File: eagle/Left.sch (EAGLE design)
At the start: 4 parts, among them J1 Rows, J2 Columns

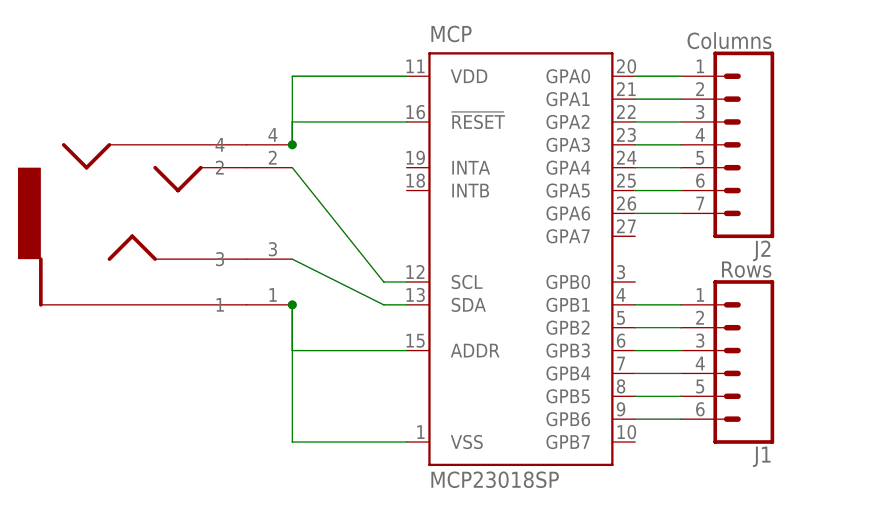
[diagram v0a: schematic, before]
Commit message: v03 of Left board
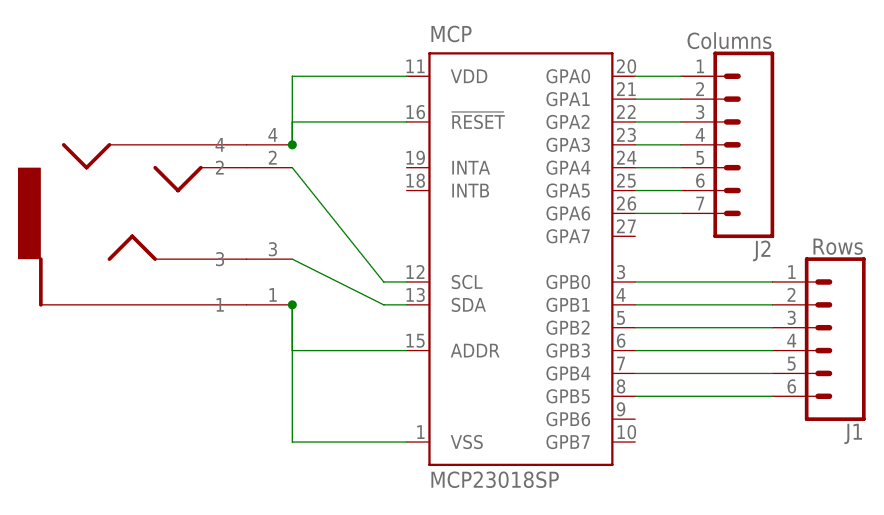
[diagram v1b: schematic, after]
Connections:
- net N$12: now also MCP.GPB0; no longer MCP.GPB1
- net N$13: now also MCP.GPB1; no longer MCP.GPB2
- net N$14: now also MCP.GPB2; no longer MCP.GPB3
- net N$15: now also MCP.GPB3; no longer MCP.GPB4
- net N$16: now also MCP.GPB4; no longer MCP.GPB5
- net N$17: now also MCP.GPB5; no longer MCP.GPB6
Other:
- moved on the sheet: J1
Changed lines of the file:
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@@
 <instance part="MCP" gate="G$1" x="25.4" y="162.56"/>
 <instance part="J2" gate="G$1" x="48.26" y="177.8" rot="R180"/>
-<instance part="J1" gate="G$1" x="48.26" y="152.4" rot="R180"/>
+<instance part="J1" gate="G$1" x="58.42" y="154.94" rot="R180"/>
 </instances>
 <busses>
@@
 <net name="N$12" class="0">
 <segment>
-<pinref part="MCP" gate="G$1" pin="GPB1"/>
+<pinref part="MCP" gate="G$1" pin="GPB0"/>
 <pinref part="J1" gate="G$1" pin="1"/>
-<wire x1="38.1" y1="157.48" x2="43.18" y2="157.48" width="0.1524" layer="91"/>
+<wire x1="38.1" y1="160.02" x2="53.34" y2="160.02" width="0.1524" layer="91"/>
 </segment>
 </net>
 <net name="N$13" class="0">
 <segment>
-<pinref part="MCP" gate="G$1" pin="GPB2"/>
+<pinref part="MCP" gate="G$1" pin="GPB1"/>
 <pinref part="J1" gate="G$1" pin="2"/>
-<wire x1="38.1" y1="154.94" x2="43.18" y2="154.94" width="0.1524" layer="91"/>
+<wire x1="38.1" y1="157.48" x2="53.34" y2="157.48" width="0.1524" layer="91"/>
 </segment>
 </net>
 <net name="N$14" class="0">
 <segment>
-<pinref part="MCP" gate="G$1" pin="GPB3"/>
+<pinref part="MCP" gate="G$1" pin="GPB2"/>
 <pinref part="J1" gate="G$1" pin="3"/>
-<wire x1="38.1" y1="152.4" x2="43.18" y2="152.4" width="0.1524" layer="91"/>
+<wire x1="38.1" y1="154.94" x2="53.34" y2="154.94" width="0.1524" layer="91"/>
 </segment>
 </net>
 <net name="N$15" class="0">
 <segment>
-<pinref part="MCP" gate="G$1" pin="GPB4"/>
+<pinref part="MCP" gate="G$1" pin="GPB3"/>
 <pinref part="J1" gate="G$1" pin="4"/>
-<wire x1="38.1" y1="149.86" x2="43.18" y2="149.86" width="0.1524" layer="91"/>
+<wire x1="38.1" y1="152.4" x2="53.34" y2="152.4" width="0.1524" layer="91"/>
 </segment>
 </net>
 <net name="N$16" class="0">
 <segment>
-<pinref part="MCP" gate="G$1" pin="GPB5"/>
+<pinref part="MCP" gate="G$1" pin="GPB4"/>
 <pinref part="J1" gate="G$1" pin="5"/>
-<wire x1="38.1" y1="147.32" x2="43.18" y2="147.32" width="0.1524" layer="91"/>
+<wire x1="38.1" y1="149.86" x2="53.34" y2="149.86" width="0.1524" layer="91"/>
 </segment>
 </net>
 <net name="N$17" class="0">
 <segment>
-<pinref part="MCP" gate="G$1" pin="GPB6"/>
+<pinref part="MCP" gate="G$1" pin="GPB5"/>
 <pinref part="J1" gate="G$1" pin="6"/>
-<wire x1="38.1" y1="144.78" x2="43.18" y2="144.78" width="0.1524" layer="91"/>
+<wire x1="38.1" y1="147.32" x2="53.34" y2="147.32" width="0.1524" layer="91"/>
 </segment>
 </net>
@@
 </sheet>
 </sheets>
-<errors>
-</errors>
 </schematic>
 </drawing>
